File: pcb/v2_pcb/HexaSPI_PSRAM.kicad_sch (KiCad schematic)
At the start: 5 parts, among them U3 APS512XXN-OB9-BG

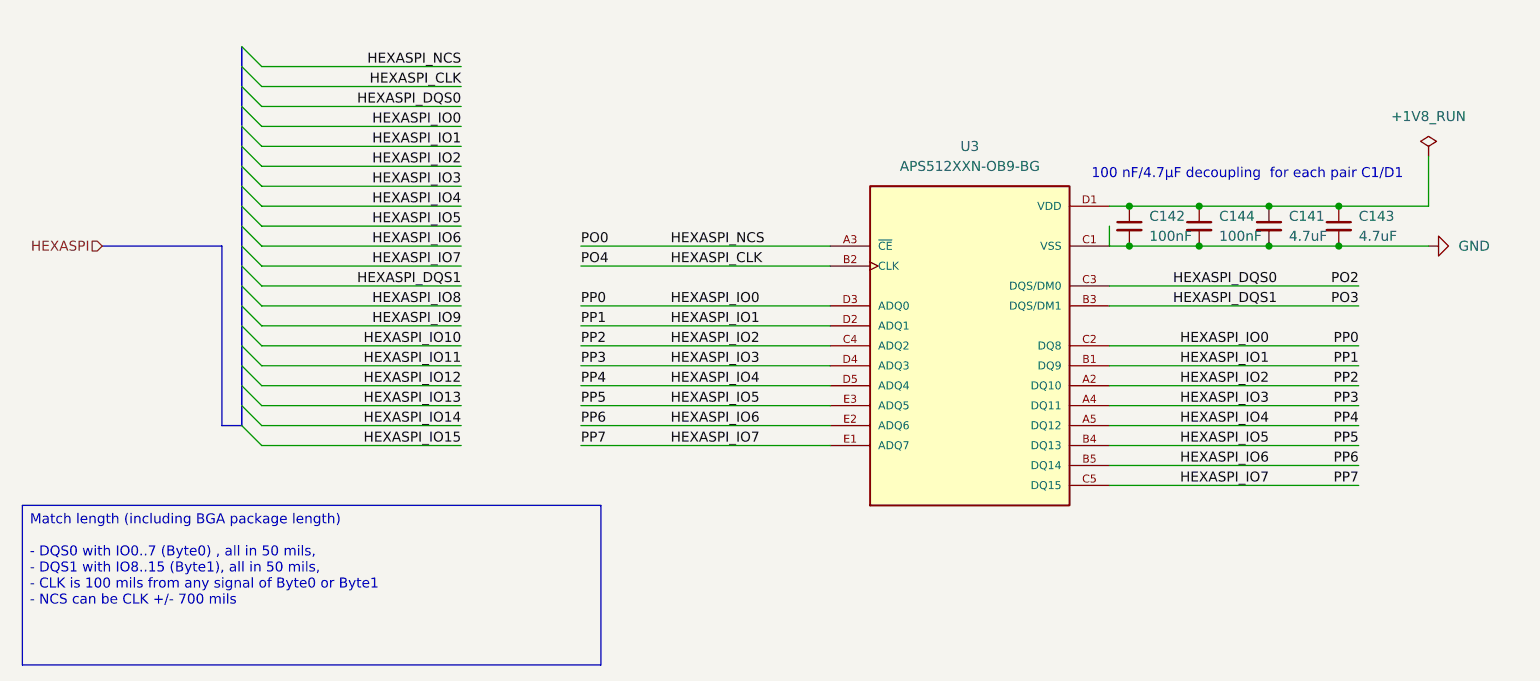
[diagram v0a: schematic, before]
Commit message: pcb done
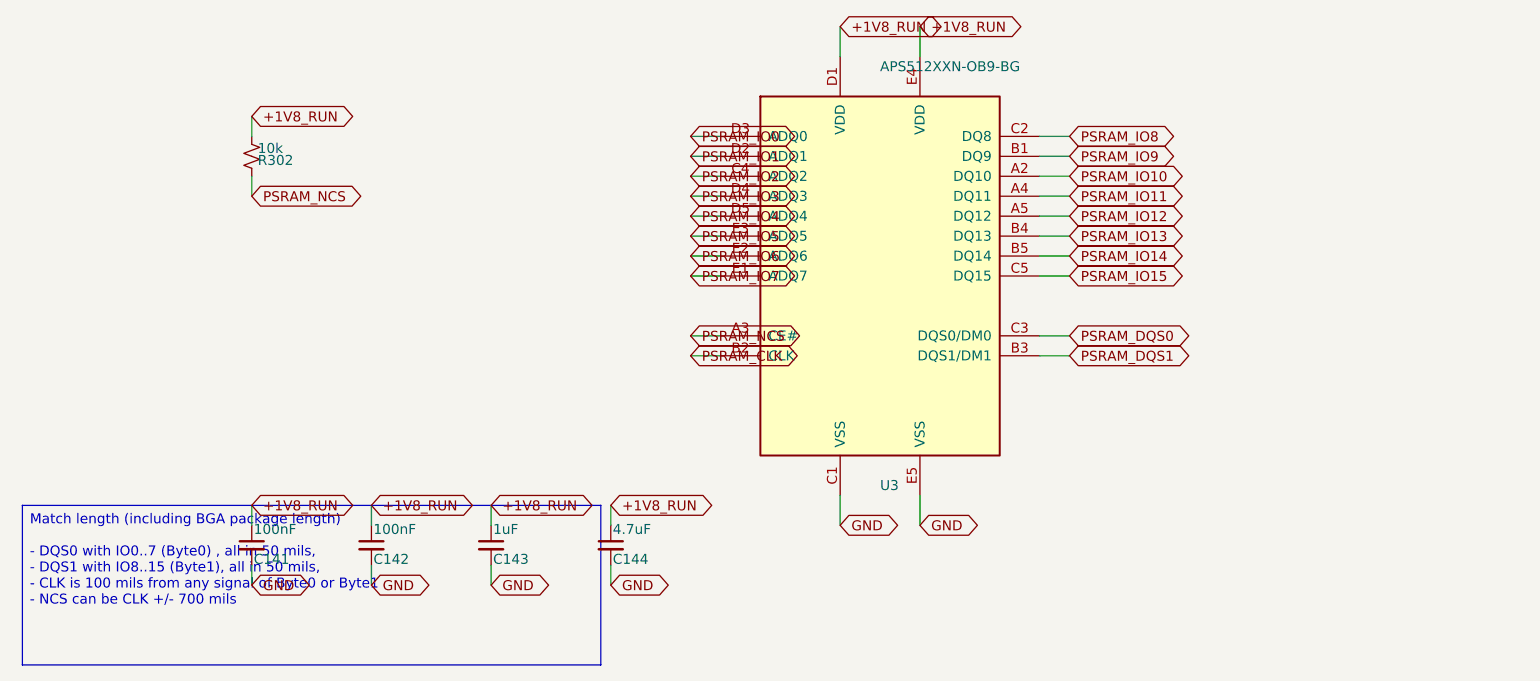
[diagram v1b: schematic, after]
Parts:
- removed U3: APS512XXN-OB9-BG, APS512XXN-OB9-BG:BGA24C100P5X5_800X600X120, symbol noob:APS256XXN-OBR-BG
- added R302: 10k, Resistor_SMD:R_0402_1005Metric, symbol Device:R_Small_US
- added U3: APS512XXN-OB9-BG, open-race-v2:WLCSP-24_6x8mm_P1.0mm_APS512XXN, symbol open-race-v2:APS512XXN-OB9-BG
- C141: value 4.7uF -> 100nF; footprint (none) -> Capacitor_SMD:C_0402_1005Metric
- C142: footprint (none) -> Capacitor_SMD:C_0402_1005Metric
- C143: value 4.7uF -> 1uF; footprint (none) -> Capacitor_SMD:C_0603_1608Metric
- C144: value 100nF -> 4.7uF; footprint (none) -> Capacitor_SMD:C_0603_1608Metric
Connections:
- net GND: now also U3.C1 (VSS), U3.E5 (VSS)
- net VDD renamed +1V8_RUN
- net +1V8_RUN: now also R302.1, U3.D1 (VDD), U3.E4 (VDD)
- new net PSRAM_CLK: U3.B2 (CLK)
- new net PSRAM_DQS0: U3.C3 (DQS0/DM0)
- new net PSRAM_DQS1: U3.B3 (DQS1/DM1)
- new net PSRAM_IO0: U3.D3 (ADQ0)
- new net PSRAM_IO1: U3.D2 (ADQ1)
- new net PSRAM_IO10: U3.A2 (DQ10)
- new net PSRAM_IO11: U3.A4 (DQ11)
- new net PSRAM_IO12: U3.A5 (DQ12)
- new net PSRAM_IO13: U3.B4 (DQ13)
- new net PSRAM_IO14: U3.B5 (DQ14)
- new net PSRAM_IO15: U3.C5 (DQ15)
- new net PSRAM_IO2: U3.C4 (ADQ2)
- new net PSRAM_IO3: U3.D4 (ADQ3)
- new net PSRAM_IO4: U3.D5 (ADQ4)
- new net PSRAM_IO5: U3.E3 (ADQ5)
- new net PSRAM_IO6: U3.E2 (ADQ6)
- new net PSRAM_IO7: U3.E1 (ADQ7)
- new net PSRAM_IO8: U3.C2 (DQ8)
- new net PSRAM_IO9: U3.B1 (DQ9)
- new net PSRAM_NCS: R302.2, U3.A3 (CE#)
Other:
- note removed: "100 nF/4.7µF decoupling for each pair C1/D1"
